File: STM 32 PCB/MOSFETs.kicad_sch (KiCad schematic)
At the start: 0 parts

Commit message: 10 dec
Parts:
- added C? (x2): 2N2, symbol Device:C
- added J? (x3): Conn_01x01_Socket, symbol Connector:Conn_01x01_Socket
- added NT? (x8): NetTie_2, symbol Device:NetTie_2
- added Q? (x6): NMOS, symbol Simulation_SPICE:NMOS
- added R? (x4): 100R, symbol Device:R
- added R? (x6): 4R7, symbol Device:R
- added R? (x3): 39K, symbol Device:R
- added R? (x2): 0R001, symbol Device:R_Shunt
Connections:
- new net: C?.2, R?.1 (x2)
- new net: NT?.2, R?.2, R?.4 (x2)
- new net: Q?.1 (D), Q?.3 (S) (x3)
- new net: NT?.2, Q?.3 (S) (x3)
- new net +VDC: Q?.1 (D), Q?.1 (D), Q?.1 (D)
- new net GND: NT?.1, NT?.1, NT?.1, R?.2, R?.2, R?.2
- new net H1_LOW: NT?.1, R?.1, R?.2
- new net H1_VS: NT?.1
- new net H2_LOW: NT?.1, R?.1, R?.2
- new net H2_VS: NT?.1
- new net H3_VS: NT?.1
- new net M_H1: R?.1
- new net M_H1_RG: Q?.2 (G), R?.2
- new net M_H2: R?.1
- new net M_H2_RG: Q?.2 (G), R?.2
- new net M_H3: R?.1
- new net M_H3_RG: Q?.2 (G), R?.2
- new net M_L1: R?.1
- new net M_L1_RG: Q?.2 (G), R?.1, R?.2
- new net M_L2: R?.1
- new net M_L2_RG: Q?.2 (G), R?.1, R?.2
- new net M_L3: R?.1
- new net M_L3_RG: Q?.2 (G), R?.1, R?.2
- new net PHASE_1: J?.1 (Pin_1), NT?.2
- new net PHASE_2: J?.1 (Pin_1), NT?.2
- new net PHASE_3: J?.1 (Pin_1), NT?.2
- new net S1_N: C?.1, C?.1, R?.1, R?.1
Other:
- note added: "Hx_VS"
- note added: "MCU SENSING FEEDBACK"
- note added: "MOSFETs"
- note added: "OUTPUT PHASE 1"
- note added: "OUTPUT PHASE 2"
- note added: "OUTPUT PHASE 3"
- note added: "PHASE 1"
- note added: "PHASE 2"
- note added: "PHASE 3"
- note added: "PLACE AS CLOSE AS POSSIBLE TO THE BULK CAPACITANCE"
- note added: "Q_CONTROL"
- note added: "SENSE 1"
- note added: "SENSE 2"

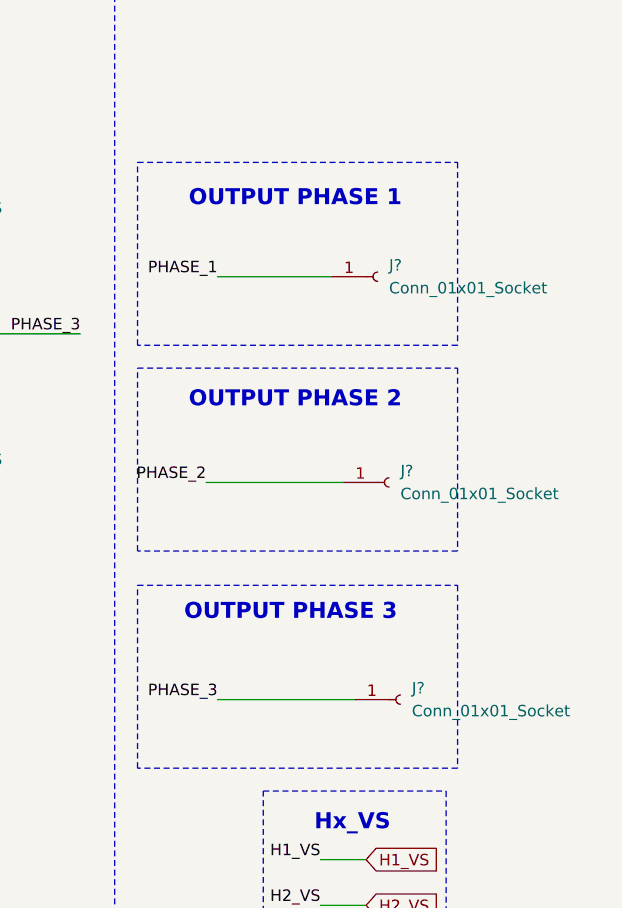
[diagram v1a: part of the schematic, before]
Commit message: 11 Dec
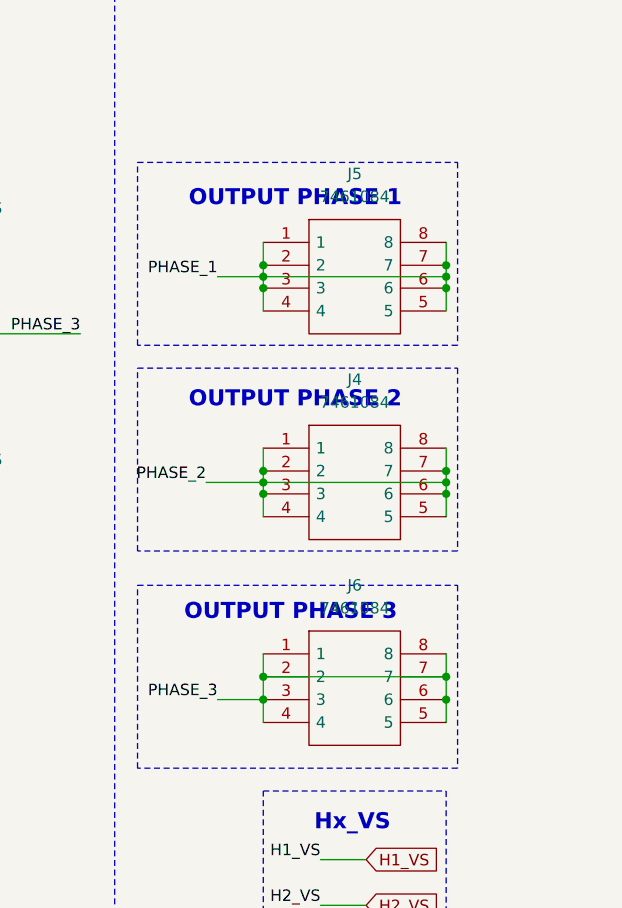
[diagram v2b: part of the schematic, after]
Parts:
- removed J? (x3): Conn_01x01_Socket, symbol Connector:Conn_01x01_Socket
- added J4, J5, J6: 7461084, 7461084, symbol 7461084:7461084
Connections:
- net PHASE_1: now also J5.1, J5.2, J5.3, J5.4, J5.5, J5.6, J5.7, J5.8
- net PHASE_2: now also J4.1, J4.2, J4.3, J4.4, J4.5, J4.6, J4.7, J4.8
- net PHASE_3: now also J6.1, J6.2, J6.3, J6.4, J6.5, J6.6, J6.7, J6.8
